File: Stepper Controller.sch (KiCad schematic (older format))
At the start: 44 parts, among them J1 FTDI, J2 ENCODER, J3 LIMIT_SWITCH, J4 ICSP, J5 MAIN_CONNECTOR, J6 Stepper, Q1 BSS138, Q2 BSS138, Q3 BSS138, Q4 BSS138, SW1 RESET, U1 ATmega328PB-MU, U2 AZ1117-5.0, Y1 16 MHz

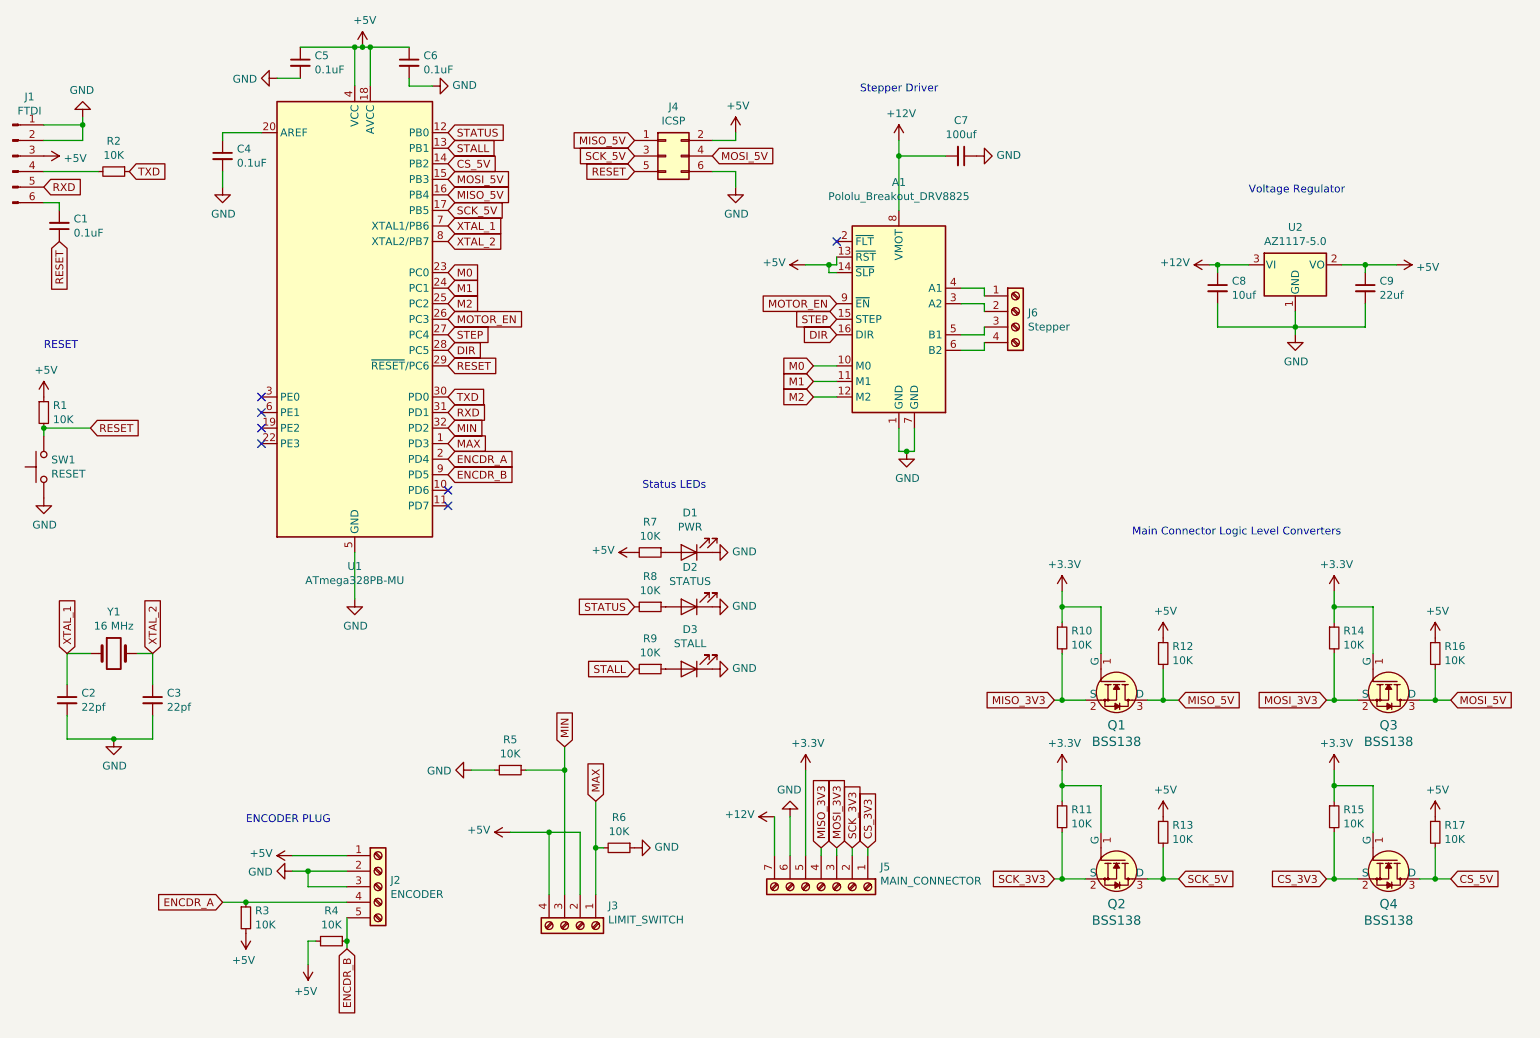
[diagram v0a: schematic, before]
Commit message: completed
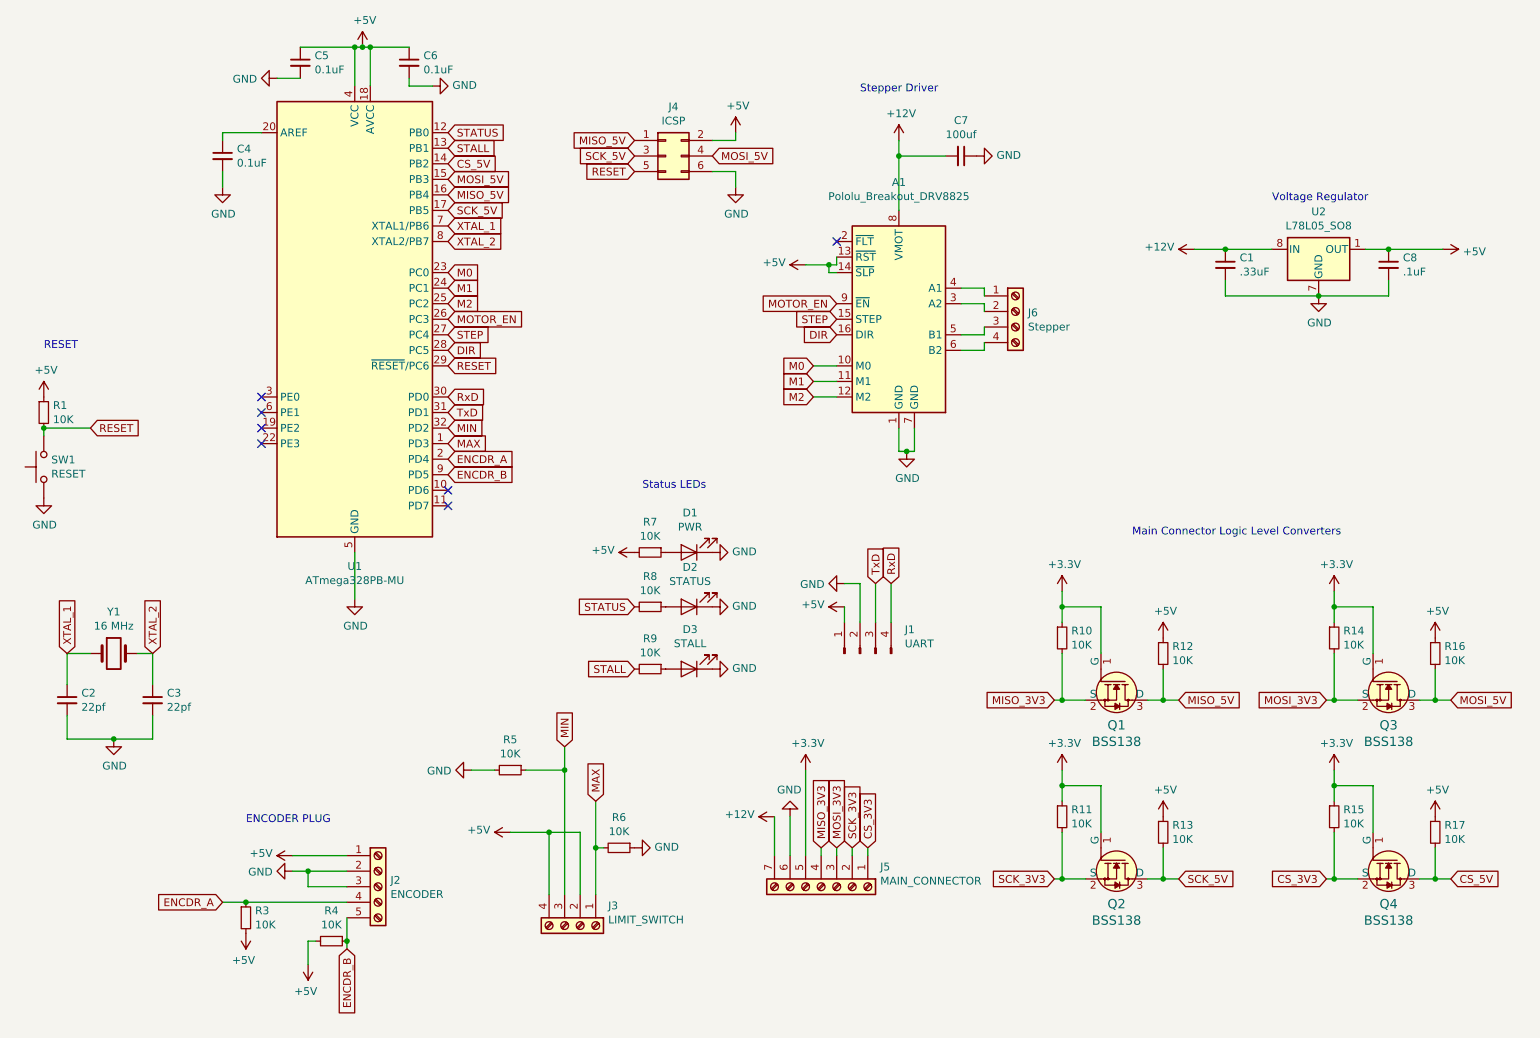
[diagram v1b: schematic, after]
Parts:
- removed C9: 22uf, Capacitor_SMD:C_0201_0603Metric, symbol Device:C_Small
- removed J1: FTDI, Connector_PinHeader_2.54mm:PinHeader_1x06_P2.54mm_Vertical, symbol Connector:Conn_01x06_Male
- removed R2: 10K, Resistor_SMD:R_0603_1608Metric, symbol Device:R_Small
- removed U2: AZ1117-5.0, Package_TO_SOT_SMD:SOT-223, symbol Regulator_Linear:AZ1117-5.0
- added J1: UART, Connector_PinHeader_2.54mm:PinHeader_1x04_P2.54mm_Vertical, symbol Connector:Conn_01x04_Male
- added U2: L78L05_SO8, Package_SO:SOIC-8_3.9x4.9mm_P1.27mm, symbol Regulator_Linear:L78L05_SO8
- C1: value 0.1uF -> .33uF; footprint Capacitor_SMD:C_0201_0603Metric -> Capacitor_SMD:C_0603_1608Metric
- C8: value 10uf -> .1uF; footprint Capacitor_SMD:C_0201_0603Metric -> Capacitor_SMD:C_0603_1608Metric
- J4: footprint Connector_PinHeader_2.54mm:PinHeader_1x06_P2.54mm_Vertical -> Connector_PinSocket_2.54mm:PinSocket_2x03_P2.54mm_Vertical
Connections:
- net +12V: now also C1.1, U2.8 (IN); no longer C8.1
- net +5V: now also C8.1, J1.1 (Pin_1), U2.1 (OUT)
- net GND: now also C1.2, J1.2 (Pin_2), U2.2 (GND), U2.3 (GND), U2.6 (GND), U2.7 (GND)
- net RESET: no longer C1.1
- net RXD renamed TxD
- net TxD: now also J1.3 (Pin_3)
- net TXD renamed RxD
- net RxD: now also J1.4 (Pin_4)
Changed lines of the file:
@@
 EESchema Schematic File Version 4
+LIBS:Stepper Controller-cache
 EELAYER 30 0
 EELAYER END
@@
 Wire Wire Line
 	5900 5900 5900 5650
-$Comp
-L Regulator_Linear:AZ1117-5.0 U2
-U 1 1 5E2EF64F
-P 9150 2100
-F 0 "U2" H 9150 2342 50  0000 C CNN
-F 1 "AZ1117-5.0" H 9150 2251 50  0000 C CNN
-F 2 "Package_TO_SOT_SMD:SOT-223" H 9150 2350 50  0001 C CIN
-F 3 "https://www.diodes.com/assets/Datasheets/AZ1117.pdf" H 9150 2100 50  0001 C CNN
-	1    9150 2100
-	1    0    0    -1
-$EndComp
-$Comp
-L power:+12V #PWR035
-U 1 1 5E2F0949
-P 8600 2100
-F 0 "#PWR035" H 8600 1950 50  0001 C CNN
-F 1 "+12V" V 8615 2228 50  0000 L CNN
-F 2 "" H 8600 2100 50  0001 C CNN
-F 3 "" H 8600 2100 50  0001 C CNN
-	1    8600 2100
-	0    -1   -1   0
-$EndComp
-Wire Wire Line
-	8600 2100 8650 2100
-$Comp
-L Device:C_Small C8
-U 1 1 5E2F177A
-P 8650 2250
-F 0 "C8" H 8742 2296 50  0000 L CNN
-F 1 "10uf" H 8742 2205 50  0000 L CNN
-F 2 "Capacitor_SMD:C_0201_0603Metric" H 8650 2250 50  0001 C CNN
-F 3 "~" H 8650 2250 50  0001 C CNN
-	1    8650 2250
-	1    0    0    -1
-$EndComp
-$Comp
-L Device:C_Small C9
-U 1 1 5E2F1C89
-P 9600 2250
-F 0 "C9" H 9692 2296 50  0000 L CNN
-F 1 "22uf" H 9692 2205 50  0000 L CNN
-F 2 "Capacitor_SMD:C_0201_0603Metric" H 9600 2250 50  0001 C CNN
-F 3 "~" H 9600 2250 50  0001 C CNN
-	1    9600 2250
-	1    0    0    -1
-$EndComp
-$Comp
-L power:+5V #PWR039
-U 1 1 5E2F2464
-P 9800 2100
-F 0 "#PWR039" H 9800 1950 50  0001 C CNN
-F 1 "+5V" V 9815 2228 50  0000 L CNN
-F 2 "" H 9800 2100 50  0001 C CNN
-F 3 "" H 9800 2100 50  0001 C CNN
-	1    9800 2100
-	0    1    1    0
-$EndComp
-Wire Wire Line
-	9450 2100 9600 2100
-Wire Wire Line
-	9600 2100 9600 2150
-Wire Wire Line
-	9600 2100 9800 2100
-Connection ~ 9600 2100
-$Comp
-L power:GND #PWR036
-U 1 1 5E2F362B
-P 9150 2550
-F 0 "#PWR036" H 9150 2300 50  0001 C CNN
-F 1 "GND" H 9155 2377 50  0000 C CNN
-F 2 "" H 9150 2550 50  0001 C CNN
-F 3 "" H 9150 2550 50  0001 C CNN
-	1    9150 2550
-	1    0    0    -1
-$EndComp
-Wire Wire Line
-	8650 2350 8650 2500
-Wire Wire Line
-	8650 2500 9150 2500
-Wire Wire Line
-	9150 2500 9150 2550
-Wire Wire Line
-	9150 2400 9150 2500
-Connection ~ 9150 2500
-Wire Wire Line
-	9150 2500 9600 2500
-Wire Wire Line
-	9600 2500 9600 2350
 $Comp
 L Device:LED D1
@@
 Text Notes 8100 3850 0    50   ~ 0
 Main Connector Logic Level Converters
-Text Notes 8850 1650 0    50   ~ 0
-Voltage Regulator
 Text Notes 6350 1000 0    50   ~ 0
 Stepper Driver
@@
 F 0 "J4" H 5150 1717 50  0000 C CNN
 F 1 "ICSP" H 5150 1626 50  0000 C CNN
-F 2 "Connector_PinHeader_2.54mm:PinHeader_1x06_P2.54mm_Vertical" H 5100 1400 50  0001 C CNN
+F 2 "Connector_PinSocket_2.54mm:PinSocket_2x03_P2.54mm_Vertical" H 5100 1400 50  0001 C CNN
 F 3 "~" H 5100 1400 50  0001 C CNN
 	1    5100 1400
@@
 Wire Wire Line
 	5550 1500 5400 1500
-$Comp
-L Connector:Conn_01x06_Male J1
-U 1 1 5E3AF966
-P 900 1400
-F 0 "J1" H 1008 1781 50  0000 C CNN
-F 1 "FTDI" H 1008 1690 50  0000 C CNN
-F 2 "Connector_PinHeader_2.54mm:PinHeader_1x06_P2.54mm_Vertical" H 900 1400 50  0001 C CNN
-F 3 "~" H 900 1400 50  0001 C CNN
-	1    900  1400
-	1    0    0    -1
-$EndComp
-$Comp
-L power:GND #PWR04
-U 1 1 5E3B0BFF
-P 1350 1150
-F 0 "#PWR04" H 1350 900 50  0001 C CNN
-F 1 "GND" H 1355 977 50  0000 C CNN
-F 2 "" H 1350 1150 50  0001 C CNN
-F 3 "" H 1350 1150 50  0001 C CNN
-	1    1350 1150
-	-1   0    0    1
-$EndComp
-Wire Wire Line
-	1100 1200 1350 1200
-Wire Wire Line
-	1350 1200 1350 1150
-Wire Wire Line
-	1100 1300 1350 1300
-Wire Wire Line
-	1350 1300 1350 1200
-Connection ~ 1350 1200
-$Comp
-L Device:R_Small R2
-U 1 1 5E3B8104
-P 1550 1500
-F 0 "R2" V 1354 1500 50  0000 C CNN
-F 1 "10K" V 1445 1500 50  0000 C CNN
-F 2 "Resistor_SMD:R_0603_1608Metric" H 1550 1500 50  0001 C CNN
-F 3 "~" H 1550 1500 50  0001 C CNN
-	1    1550 1500
-	0    1    1    0
-$EndComp
-Text GLabel 1650 1500 2    50   Input ~ 0
-TXD
-Text GLabel 1100 1600 2    50   Input ~ 0
-RXD
-$Comp
-L power:+5V #PWR01
-U 1 1 5E3C67FF
-P 1100 1400
-F 0 "#PWR01" H 1100 1250 50  0001 C CNN
-F 1 "+5V" V 1115 1528 50  0000 L CNN
-F 2 "" H 1100 1400 50  0001 C CNN
-F 3 "" H 1100 1400 50  0001 C CNN
-	1    1100 1400
-	0    1    1    0
-$EndComp
-Wire Wire Line
-	1450 1500 1100 1500
-$Comp
-L Device:C_Small C1
-U 1 1 5E3CA770
-P 1200 1850
-F 0 "C1" H 1108 1804 50  0000 R CNN
-F 1 "0.1uF" H 1108 1895 50  0000 R CNN
-F 2 "Capacitor_SMD:C_0201_0603Metric" H 1200 1850 50  0001 C CNN
-F 3 "~" H 1200 1850 50  0001 C CNN
-	1    1200 1850
-	-1   0    0    1
-$EndComp
-Wire Wire Line
-	1100 1700 1200 1700
-Wire Wire Line
-	1200 1700 1200 1750
-Text GLabel 1200 1950 3    50   Input ~ 0
-RESET
 $Comp
 L power:+5V #PWR013
@@
 Text Notes 1100 2650 0    50   ~ 0
 RESET
-Text GLabel 3700 2950 2    50   Input ~ 0
-TXD
-Text GLabel 3700 3050 2    50   Input ~ 0
-RXD
 Text GLabel 3700 2150 2    50   Input ~ 0
 M0
@@
 NoConn ~ 2500 2950
 Wire Wire Line
-	8650 2150 8650 2100
-Connection ~ 8650 2100
-Wire Wire Line
-	8650 2100 8850 2100
-Wire Wire Line
 	6200 5850 6200 5900
 Wire Wire Line
@@
 Wire Wire Line
 	6400 5850 6400 5900
+$Comp
+L Regulator_Linear:L78L05_SO8 U2
+U 1 1 5E3A9A16
+P 9300 2000
+F 0 "U2" H 9300 2242 50  0000 C CNN
+F 1 "L78L05_SO8" H 9300 2151 50  0000 C CNN
+F 2 "Package_SO:SOIC-8_3.9x4.9mm_P1.27mm" H 9400 2200 50  0001 C CIN
+F 3 "http://www.st.com/content/ccc/resource/technical/document/datasheet/15/55/e5/aa/23/5b/43/fd/CD00000446.pdf/files/CD00000446.pdf/jcr:content/translations/en.CD00000446.pdf" H 9500 2000 50  0001 C CNN
+	1    9300 2000
+	1    0    0    -1
+$EndComp
+$Comp
+L Device:C_Small C8
+U 1 1 5E3B0417
+P 9750 2100
+F 0 "C8" H 9842 2146 50  0000 L CNN
+F 1 ".1uF" H 9842 2055 50  0000 L CNN
+F 2 "Capacitor_SMD:C_0603_1608Metric" H 9750 2100 50  0001 C CNN
+F 3 "~" H 9750 2100 50  0001 C CNN
+	1    9750 2100
+	1    0    0    -1
+$EndComp
+$Comp
+L Device:C_Small C1
+U 1 1 5E3B0ED4
+P 8700 2100
+F 0 "C1" H 8792 2146 50  0000 L CNN
+F 1 ".33uF" H 8792 2055 50  0000 L CNN
+F 2 "Capacitor_SMD:C_0603_1608Metric" H 8700 2100 50  0001 C CNN
+F 3 "~" H 8700 2100 50  0001 C CNN
+	1    8700 2100
+	1    0    0    -1
+$EndComp
+Wire Wire Line
+	9600 2000 9750 2000
+Wire Wire Line
+	9750 2200 9750 2300
+Wire Wire Line
+	9750 2300 9300 2300
+Wire Wire Line
+	9000 2000 8700 2000
+Wire Wire Line
+	8700 2200 8700 2300
+Wire Wire Line
+	8700 2300 9300 2300
+Connection ~ 9300 2300
+$Comp
+L power:GND #PWR0101
+U 1 1 5E3C7FBB
+P 9300 2300
+F 0 "#PWR0101" H 9300 2050 50  0001 C CNN
+F 1 "GND" H 9305 2127 50  0000 C CNN
+F 2 "" H 9300 2300 50  0001 C CNN
+F 3 "" H 9300 2300 50  0001 C CNN
+	1    9300 2300
+	1    0    0    -1
+$EndComp
+$Comp
+L power:+5V #PWR0102
+U 1 1 5E3C93B1
+P 10100 2000
+F 0 "#PWR0102" H 10100 1850 50  0001 C CNN
+F 1 "+5V" V 10115 2128 50  0000 L CNN
+F 2 "" H 10100 2000 50  0001 C CNN
+F 3 "" H 10100 2000 50  0001 C CNN
+	1    10100 2000
+	0    1    1    0
+$EndComp
+Wire Wire Line
+	9750 2000 10100 2000
+Connection ~ 9750 2000
+$Comp
+L power:+12V #PWR0103
+U 1 1 5E3CFA4A
+P 8500 2000
+F 0 "#PWR0103" H 8500 1850 50  0001 C CNN
+F 1 "+12V" V 8515 2128 50  0000 L CNN
+F 2 "" H 8500 2000 50  0001 C CNN
+F 3 "" H 8500 2000 50  0001 C CNN
+	1    8500 2000
+	0    -1   -1   0
+$EndComp
+Wire Wire Line
+	8500 2000 8700 2000
+Connection ~ 8700 2000
+Text Notes 9000 1700 0    50   ~ 0
+Voltage Regulator
+Text GLabel 3700 2950 2    50   Input ~ 0
+RxD
+Text GLabel 3700 3050 2    50   Input ~ 0
+TxD
+$Comp
+L Connector:Conn_01x04_Male J1
+U 1 1 5E45F4DE
+P 6350 4600
+F 0 "J1" V 6504 4312 50  0000 R CNN
+F 1 "UART" V 6413 4312 50  0000 R CNN
+F 2 "Connector_PinHeader_2.54mm:PinHeader_1x04_P2.54mm_Vertical" H 6350 4600 50  0001 C CNN
+F 3 "~" H 6350 4600 50  0001 C CNN
+	1    6350 4600
+	0    -1   -1   0
+$EndComp
+$Comp
+L power:GND #PWR0104
+U 1 1 5E460610
+P 6250 4150
+F 0 "#PWR0104" H 6250 3900 50  0001 C CNN
+F 1 "GND" V 6255 4022 50  0000 R CNN
+F 2 "" H 6250 4150 50  0001 C CNN
+F 3 "" H 6250 4150 50  0001 C CNN
+	1    6250 4150
+	0    1    1    0
+$EndComp
+$Comp
+L power:+5V #PWR0105
+U 1 1 5E461A3B
+P 6250 4300
+F 0 "#PWR0105" H 6250 4150 50  0001 C CNN
+F 1 "+5V" V 6265 4428 50  0000 L CNN
+F 2 "" H 6250 4300 50  0001 C CNN
+F 3 "" H 6250 4300 50  0001 C CNN
+	1    6250 4300
+	0    -1   -1   0
+$EndComp
+Wire Wire Line
+	6250 4300 6250 4400
+Wire Wire Line
+	6350 4400 6350 4150
+Wire Wire Line
+	6350 4150 6250 4150
+Text GLabel 6450 4150 1    50   Input ~ 0
+TxD
+Text GLabel 6550 4150 1    50   Input ~ 0
+RxD
+Wire Wire Line
+	6550 4150 6550 4400
+Wire Wire Line
+	6450 4150 6450 4400
 $EndSCHEMATC
